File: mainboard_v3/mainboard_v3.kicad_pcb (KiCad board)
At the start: 4 copper layers, 156.9 x 46 mm, 38 parts, among them J1 PWR_IN, J2 CLK_IN, J3 Conn_01x50, SW1 RESET, U1 DS1813, U2 W65C02SxP, U3 74HC21, U4 CY62256-70PC, U5 28C256, U6 74HC133, U7 74HC04, U8 74HC00, U9 74HC138, X1 ACO-xxxMHz

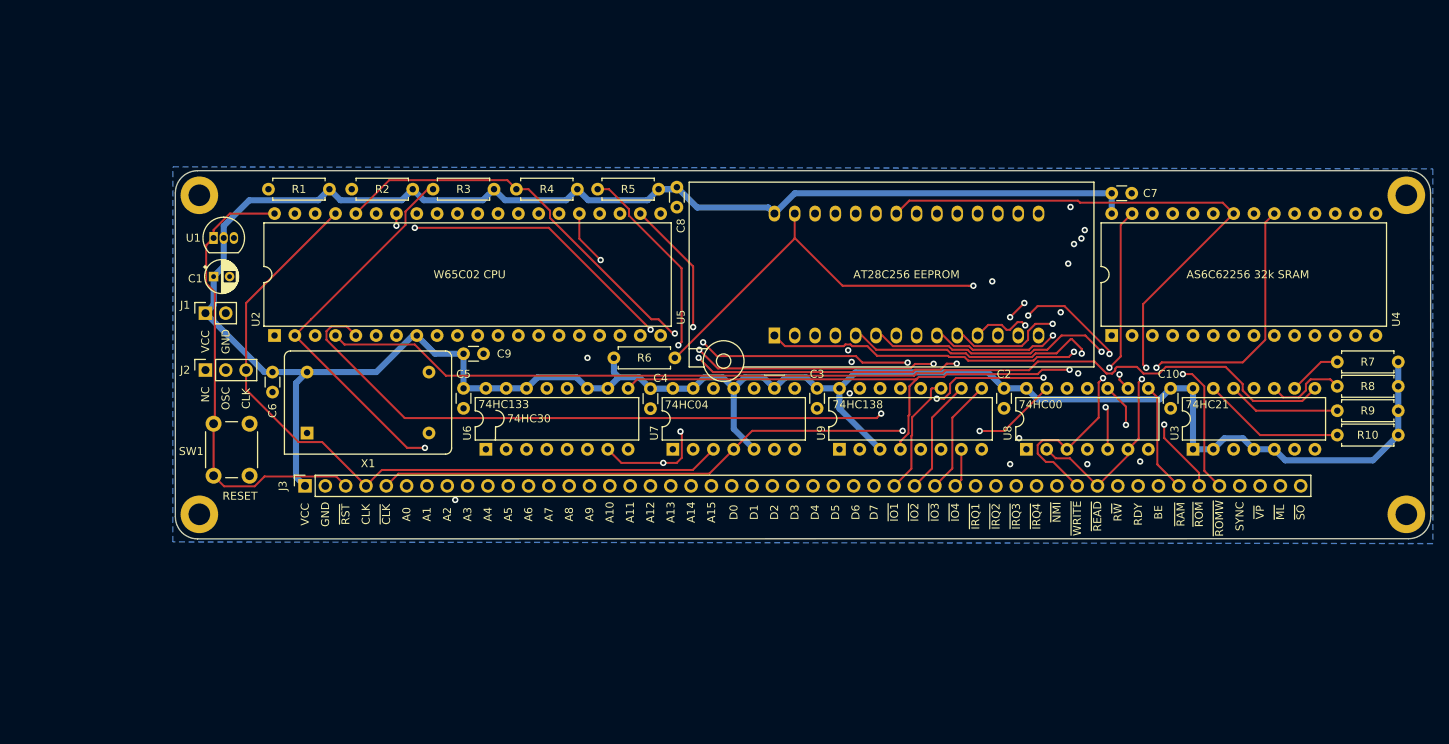
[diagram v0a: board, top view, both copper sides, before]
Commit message: Mainboard v3
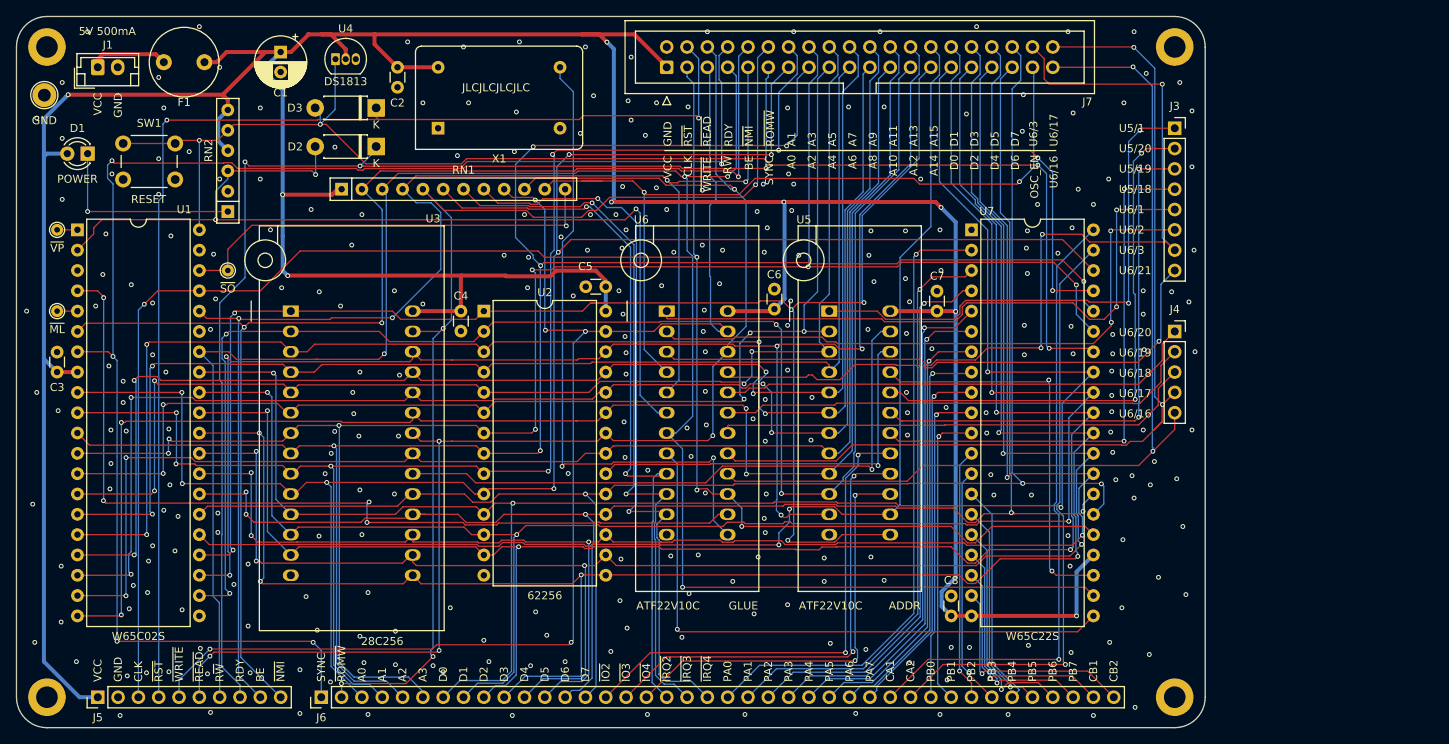
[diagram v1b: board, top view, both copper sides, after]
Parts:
- removed C10, C9: 0.1uF, Capacitor_THT:C_Disc_D3.0mm_W1.6mm_P2.50mm
- removed J2: CLK_IN, Connector_PinSocket_2.54mm:PinSocket_1x03_P2.54mm_Vertical
- removed R1, R10, R2, R3, R4, R5, R6, R7, R8, R9: 10K, Resistor_THT:R_Axial_DIN0207_L6.3mm_D2.5mm_P7.62mm_Horizontal
- removed U8: 74HC00, Package_DIP:DIP-14_W7.62mm
- removed U9: 74HC138, Package_DIP:DIP-16_W7.62mm
- added D1: POWER, LED_THT:LED_D3.0mm, F.Cu at (47.0, 79.4)
- added D2: 1N5817, Diode_THT:D_DO-41_SOD81_P7.62mm_Horizontal, F.Cu at (83.1, 78.5)
- added D3: 1N5817, Diode_THT:D_DO-41_SOD81_P7.62mm_Horizontal, F.Cu at (83.1, 73.7)
- added F1: 500mA, Fuse:Fuse_Littelfuse_372_D8.50mm, F.Cu at (61.6, 67.9)
- added J4: PLD, Connector_PinSocket_2.54mm:PinSocket_1x05_P2.54mm_Vertical, F.Cu at (182.9, 101.6)
- added J5: IO, Connector_PinHeader_2.54mm:PinHeader_1x10_P2.54mm_Vertical, F.Cu at (48.3, 147.3)
- added J6: IO, Connector_PinHeader_2.54mm:PinHeader_1x40_P2.54mm_Vertical, F.Cu at (76.2, 147.3)
- added J7: DEBUG, Connector_IDC:IDC-Header_2x20_P2.54mm_Vertical, F.Cu at (119.4, 68.6)
- added RN1: 10k, Resistor_THT:R_Array_SIP12, F.Cu at (78.7, 83.8)
- added RN2: 1k, Resistor_THT:R_Array_SIP6, F.Cu at (64.5, 86.6)
- added TP1: GND, TestPoint:TestPoint_Loop_D2.60mm_Drill1.6mm_Beaded, F.Cu at (41.6, 72.1)
- added TP2: ~ML, TestPoint:TestPoint_THTPad_D1.5mm_Drill0.7mm, F.Cu at (43.2, 99.1)
- added TP3: ~VP, TestPoint:TestPoint_THTPad_D1.5mm_Drill0.7mm, F.Cu at (43.2, 88.9)
- added TP4: ~SO, TestPoint:TestPoint_THTPad_D1.5mm_Drill0.7mm, F.Cu at (64.5, 94.0)
- C1: value 1uF -> 10uF; footprint Capacitor_THT:CP_Radial_D4.0mm_P2.00mm -> Capacitor_THT:CP_Radial_D6.3mm_P2.50mm
- J1: footprint Connector_PinSocket_2.54mm:PinSocket_1x02_P2.54mm_Vertical -> Connector_JST:JST_EH_B2B-EH-A_1x02_P2.50mm_Vertical
- J3: value Conn_01x50 -> PLD; footprint AK's_Footprints:PinSocket_1x50_P2.54mm_Vertical -> Connector_PinSocket_2.54mm:PinSocket_1x08_P2.54mm_Vertical
- U1: value DS1813 -> W65C02SxP; footprint Package_TO_SOT_THT:TO-92_Inline -> Package_DIP:DIP-40_W15.24mm
- U2: value W65C02SxP -> CY62256-70PC; footprint Package_DIP:DIP-40_W15.24mm -> Package_DIP:DIP-28_W15.24mm
- U3: value 74HC21 -> 28C256; footprint Package_DIP:DIP-14_W7.62mm -> Socket:DIP_Socket-28_W11.9_W12.7_W15.24_W17.78_W18.5_3M_228-1277-00-0602J
- U4: value CY62256-70PC -> DS1813; footprint Package_DIP:DIP-28_W15.24mm -> Package_TO_SOT_THT:TO-92_Inline
- U5: value 28C256 -> ATF22V10C; footprint Socket:DIP_Socket-28_W11.9_W12.7_W15.24_W17.78_W18.5_3M_228-1277-00-0602J -> Socket:DIP_Socket-24_W4.3_W5.08_W7.62_W10.16_W10.9_3M_224-5248-00-0602J
- U6: value 74HC133 -> ATF22V10C; footprint Package_DIP:DIP-16_W7.62mm -> Socket:DIP_Socket-24_W4.3_W5.08_W7.62_W10.16_W10.9_3M_224-5248-00-0602J
- U7: value 74HC04 -> W65C22SxP; footprint Package_DIP:DIP-14_W7.62mm -> Package_DIP:DIP-40_W15.24mm
- X1: value ACO-xxxMHz -> 4Mhz
- moved H3 171.5 mm to (41.9, 147.3)
- moved H1 170.9 mm to (41.9, 66.0)
- moved H4 124.0 mm to (182.9, 147.3)
- moved H2 123.3 mm to (182.9, 66.0)
- moved J3 117.5 mm to (182.9, 76.2), turned to 0 degrees
- moved U3 114.1 mm to (72.4, 99.1), turned to 0 degrees
- moved U4 103.0 mm to (78.0, 67.6), turned to 0 degrees
- moved C3 95.0 mm to (43.2, 106.7), turned to 90 degrees
- moved C2 85.8 mm to (85.7, 68.6)
- moved C8 63.6 mm to (154.9, 137.2), turned to 90 degrees
- moved C6 63.2 mm to (132.8, 98.8), turned to 90 degrees
- moved U7 46.3 mm to (157.5, 88.9), turned to 0 degrees
- moved SW1 43.0 mm to (51.4, 78.1), turned to 0 degrees
- moved X1 41.5 mm to (90.8, 76.2)
- moved J1 33.6 mm to (48.3, 68.6), turned to 0 degrees
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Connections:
- J1 pad 1: VCC -> Net-(F1-Pad2)
- J3 pad 1: VCC -> U5-1
- J3 pad 2: GND -> U5-20
- J3 pad 3: RST -> U5-19
- J3 pad 4: CLK -> U5-18
- J3 pad 5: ~CLK -> U6-1
- J3 pad 6: /a0 -> U6-2
- J3 pad 7: /a1 -> U6-3
- J3 pad 8: /a2 -> U6-21
- U1 pad 1: RST -> Net-(TP3-Pad1)
- U1 pad 2: VCC -> RDY
- U1 pad 3: GND -> Net-(U1-Pad3)
- U2 pad 1: VP -> /a14
- U2 pad 10: /a1 -> /a0
- U2 pad 11: /a2 -> /d0
- U2 pad 12: /a3 -> /d1
- U2 pad 13: /a4 -> /d2
- U2 pad 14: /a5 -> GND
- U2 pad 15: /a6 -> /d3
- U2 pad 16: /a7 -> /d4
- U2 pad 17: /a8 -> /d5
- U2 pad 18: /a9 -> /d6
- U2 pad 19: /a10 -> /d7
- U2 pad 2: RDY -> /a12
- U2 pad 20: /a11 -> RAM_~CS
- U2 pad 21: GND -> /a10
- U2 pad 22: /a12 -> ~READ
- U2 pad 23: /a13 -> /a11
- U2 pad 24: /a14 -> /a9
- U2 pad 25: /a15 -> /a8
- U2 pad 26: /d7 -> /a13
- U2 pad 27: /d6 -> ~WRITE
- U2 pad 28: /d5 -> VCC
- U2 pad 3: (no net) -> /a7
- U2 pad 4: IRQ -> /a6
- U2 pad 5: ML -> /a5
- U2 pad 6: NMI -> /a4
- U2 pad 7: SYNC -> /a3
- U2 pad 8: VCC -> /a2
- U2 pad 9: /a0 -> /a1
- U3 pad 1: VCC -> /a14
- U3 pad 10: IRQ2 -> /a0
- U3 pad 11: (no net) -> /d0
- U3 pad 12: IRQ3 -> /d1
- U3 pad 13: IRQ4 -> /d2
- U3 pad 14: VCC -> GND
- U3 pad 2: VCC -> /a12
- U3 pad 3: (no net) -> /a7
- U3 pad 4: VCC -> /a6
- U3 pad 5: VCC -> /a5
- U3 pad 6: (no net) -> /a4
- U3 pad 7: GND -> /a3
- U3 pad 8: IRQ -> /a2
- U3 pad 9: IRQ1 -> /a1
- U4 pad 1: /a14 -> RST
- U4 pad 2: /a12 -> VCC
- U4 pad 3: /a7 -> GND
- U5 pad 1: /a14 -> U5-1
- U5 pad 10: /a0 -> /a12
- U5 pad 11: /d0 -> /a13
- U5 pad 12: /d1 -> GND
- U5 pad 13: /d2 -> /a14
- U5 pad 14: GND -> /a15
- U5 pad 15: /d3 -> IO4
- U5 pad 16: /d4 -> IO3
- U5 pad 17: /d5 -> IO2
- U5 pad 18: /d6 -> U5-18
- U5 pad 19: /d7 -> U5-19
- U5 pad 2: /a12 -> /a4
- U5 pad 20: ROM_~CS -> U5-20
- U5 pad 21: /a10 -> IO1
- U5 pad 22: ~READ -> RAM_~CS
- U5 pad 23: /a11 -> ROM_~CS
- U5 pad 24: /a9 -> VCC
- U5 pad 3: /a7 -> /a5
- U5 pad 5: /a5 -> /a7
- U5 pad 6: /a4 -> /a8
- U5 pad 7: /a3 -> /a9
- U5 pad 8: /a2 -> /a10
- U5 pad 9: /a1 -> /a11
- U6 pad 1: /a6 -> U6-1
- U6 pad 10: VCC -> IRQ3
- U6 pad 11: VCC -> IRQ4
- U6 pad 12: /a13 -> GND
- U6 pad 13: /a14 -> OSC
- U6 pad 14: VCC -> IRQ
- U6 pad 15: VCC -> CLK
- U6 pad 16: VCC -> U6-16
- U6 pad 2: /a7 -> U6-2
- U6 pad 3: /a8 -> U6-3
- U6 pad 4: /a9 -> OSC_EN
- U6 pad 5: /a10 -> BE
- U6 pad 6: /a11 -> RDY
- U6 pad 7: /a12 -> RW
- U6 pad 8: GND -> IRQ1
- U6 pad 9: Net-(U6-Pad9) -> IRQ2
- U7 pad 1: /a15 -> GND
- U7 pad 10: (no net) -> PB0
- U7 pad 11: VCC -> PB1
- U7 pad 12: (no net) -> PB2
- U7 pad 13: VCC -> PB3
- U7 pad 14: VCC -> PB4
- U7 pad 2: ROM_~CS -> PA0
- U7 pad 3: CLK -> PA1
- U7 pad 4: ~CLK -> PA2
- U7 pad 5: VCC -> PA3
- U7 pad 6: (no net) -> PA4
- U7 pad 7: GND -> PA5
- U7 pad 8: (no net) -> PA6
- U7 pad 9: VCC -> PA7
- X1 pad 1: (no net) -> Net-(X1-Pad1)
- X1 pad 8: Net-(J2-Pad2) -> OSC
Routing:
- net SO: track 155.6 -> 0.00 mm, vias 3 -> 0
- net RST_I: track 0.00 -> 150.4 mm, vias 0 -> 2
- net RDY_I: track 0.00 -> 148.3 mm, vias 0 -> 3
- net CLK: track 91.9 -> 230.0 mm, vias 0 -> 4
- net VP: track 137.7 -> 0.00 mm
- net ML: track 133.1 -> 0.00 mm, vias 3 -> 0
- net RW: track 124.6 -> 254.5 mm, vias 9 -> 4
- net ~WRITE: track 44.9 -> 172.9 mm, vias 2 -> 5
- net /a2: track 126.4 -> 253.8 mm, vias 0 -> 6
- net U6-3: track 0.00 -> 121.1 mm, vias 0 -> 3
- net U6-16: track 0.00 -> 120.2 mm, vias 0 -> 2
- net U6-17: track 0.00 -> 118.9 mm, vias 0 -> 2
- net RST: track 58.1 -> 169.6 mm, vias 0 -> 4
- net /a0: track 139.6 -> 250.6 mm, vias 1 -> 7
- net /a15: track 43.8 -> 153.1 mm
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- added copper zone on In1.Cu, net GND
- added copper zone on In2.Cu, net GND
- removed copper zone on B.Cu, net GND
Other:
- board size 156.9 x 46 mm -> 148.6 x 88.9 mm
- net class Default: clearance 0.2 -> 0.15; trace_width 0.25 -> 0.15; via_dia 0.8 -> 0.6; via_drill 0.4 -> 0.35
- rule trace_clearance: 0.2 -> 0.15
- rule trace_min: 0.2 -> 0.15
- rule via_min_drill: 0.3 -> 0.2
- board text added: "28C256"
- board text added: "5V 500mA"
- board text added: "62256"
- board text added: "6502 Motherboard v3 2021-10-29 Adrien Kohlbecker"
- board text added: "ADDR"
- board text added: "ATF22V10C"
- board text added: "CA1"
- board text added: "CA2"
- board text added: "CB1"
- board text added: "CB2"
- board text added: "DS1813"
- board text added: "GLUE"
- board text added: "JLCJLCJLCJLC"
- board text added: "OSC_EN"
- board text added: "PA0"
- board text added: "PA1"
- board text added: "PA2"
- board text added: "PA3"
- board text added: "PA4"
- board text added: "PA5"
- board text added: "PA6"
- board text added: "PA7"
- board text added: "PB0"
- board text added: "PB1"
- board text added: "PB2"
- board text added: "PB3"
- board text added: "PB4"
- board text added: "PB5"
- board text added: "PB6"
- board text added: "PB7"
- board text added: "U5/1"
- board text added: "U5/18"
- board text added: "U5/19"
- board text added: "U5/20"
- board text added: "U6/1"
- board text added: "U6/16"
- board text added: "U6/17"
- board text added: "U6/18"
- board text added: "U6/19"
- board text added: "U6/2"
- board text added: "U6/20"
- board text added: "U6/21"
- board text added: "U6/3"
- board text added: "W65C02S"
- board text added: "W65C22S"
- board text removed: "6502 motherboard v02 2021-05-12 Adrien Kohlbecker Inspired by Ben Eater"
- board text removed: "74HC00"
- board text removed: "74HC04"
- board text removed: "74HC133"
- board text removed: "74HC138"
- board text removed: "74HC21"
- board text removed: "74HC30"
- board text removed: "AS6C62256 32k SRAM"
- board text removed: "AT28C256 EEPROM"
- board text removed: "NC"
- board text removed: "OSC"
- board text removed: "RESET"
- board text removed: "W65C02 CPU"
- board text removed: "~CLK"
- board text removed: "~IO1"
- board text removed: "~IRQ1"
- board text removed: "~ML"
- board text removed: "~RAM"
- board text removed: "~ROM"
- board text removed: "~SO"
- board text removed: "~VP"
